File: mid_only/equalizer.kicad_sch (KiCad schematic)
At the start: 22 parts, among them J1 Conn_01x04_Socket, J2 Conn_01x04_Socket, U105 TL072

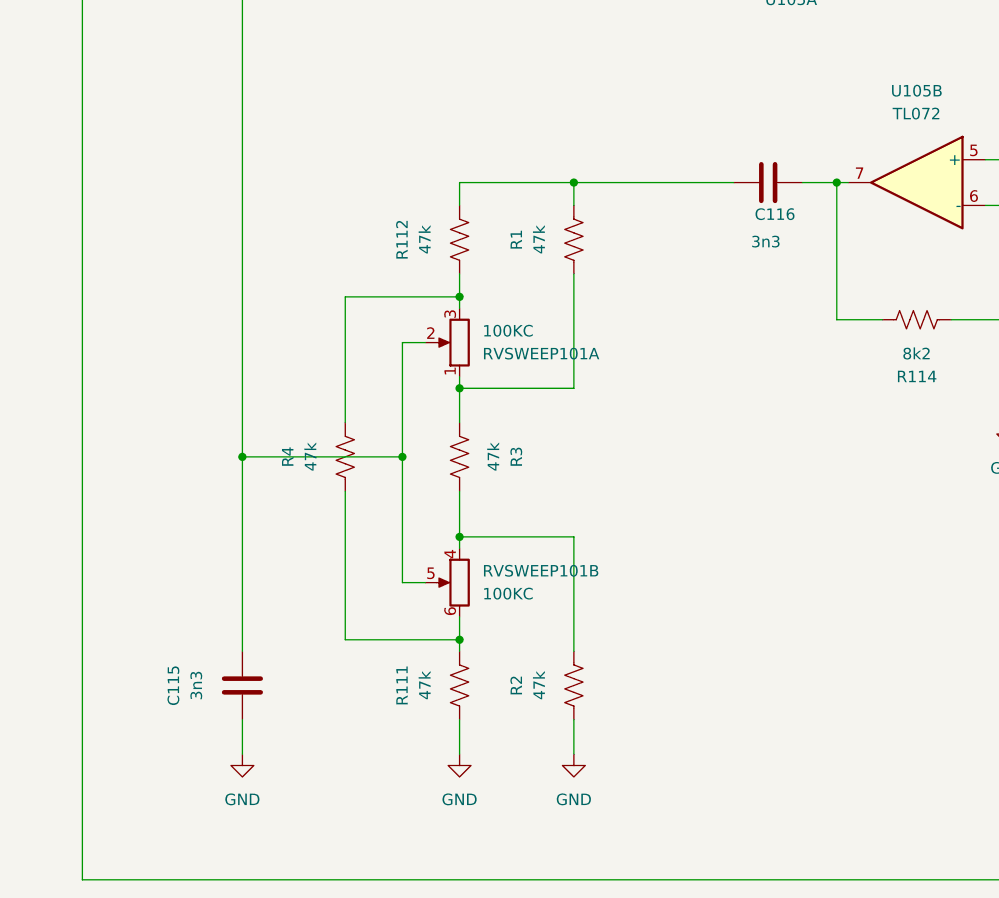
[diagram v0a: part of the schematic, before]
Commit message: med ok
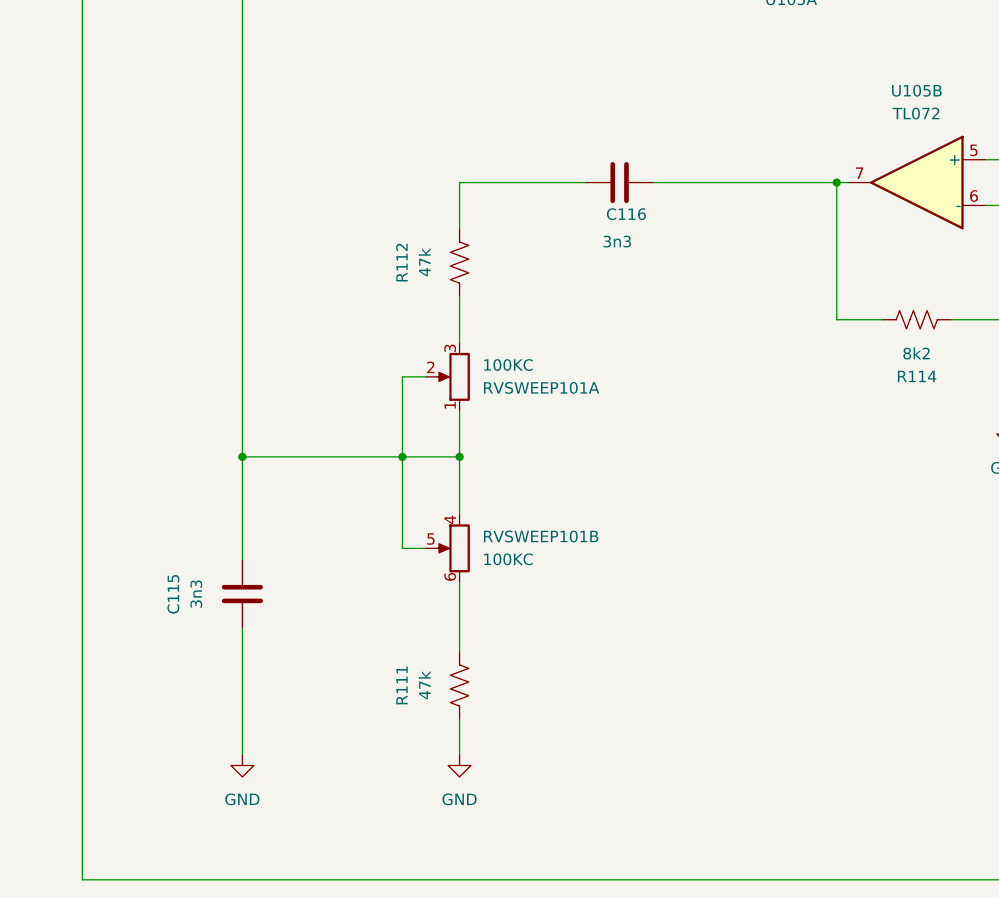
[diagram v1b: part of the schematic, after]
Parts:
- removed R1, R2, R3, R4: 47k, Resistor_THT:R_Axial_DIN0207_L6.3mm_D2.5mm_P10.16mm_Horizontal, symbol Device:R_US
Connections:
- net at C115.2, RVSWEEP101.2, RVSWEEP101.5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: now also RVSWEEP101.1, RVSWEEP101.4
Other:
- moved on the sheet: C115, C116, R112, RVSWEEP101A, RVSWEEP101B
